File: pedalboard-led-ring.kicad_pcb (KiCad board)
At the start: 2 copper layers, 24 x 24 mm, 33 parts, among them J1 middle, J2 edge

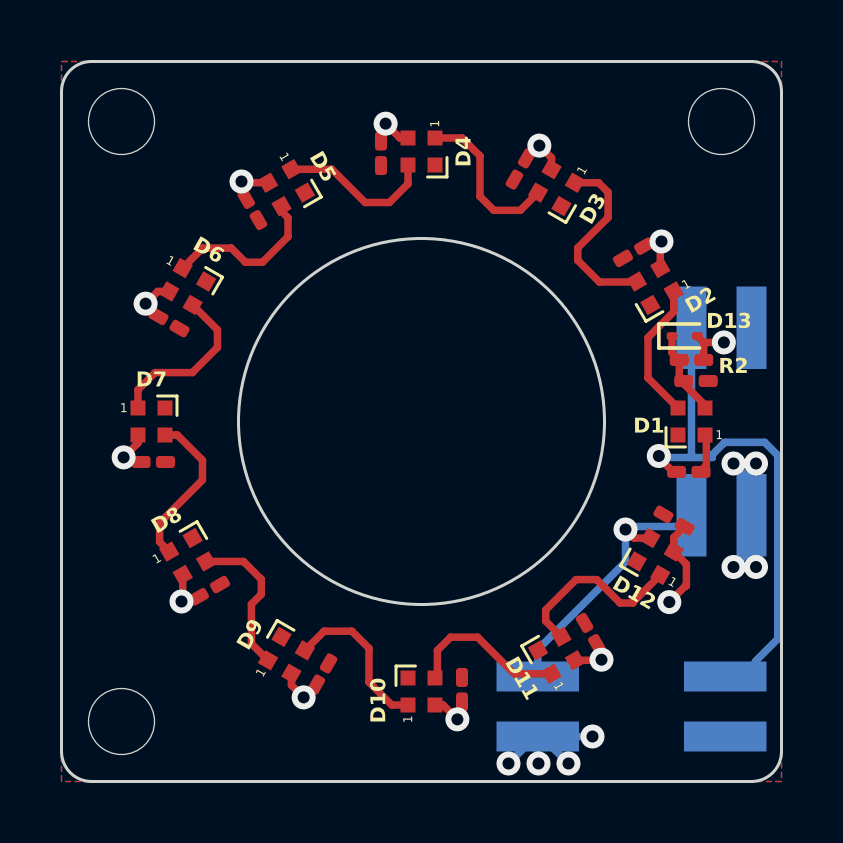
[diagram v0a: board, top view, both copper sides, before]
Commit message: Simplificaitons
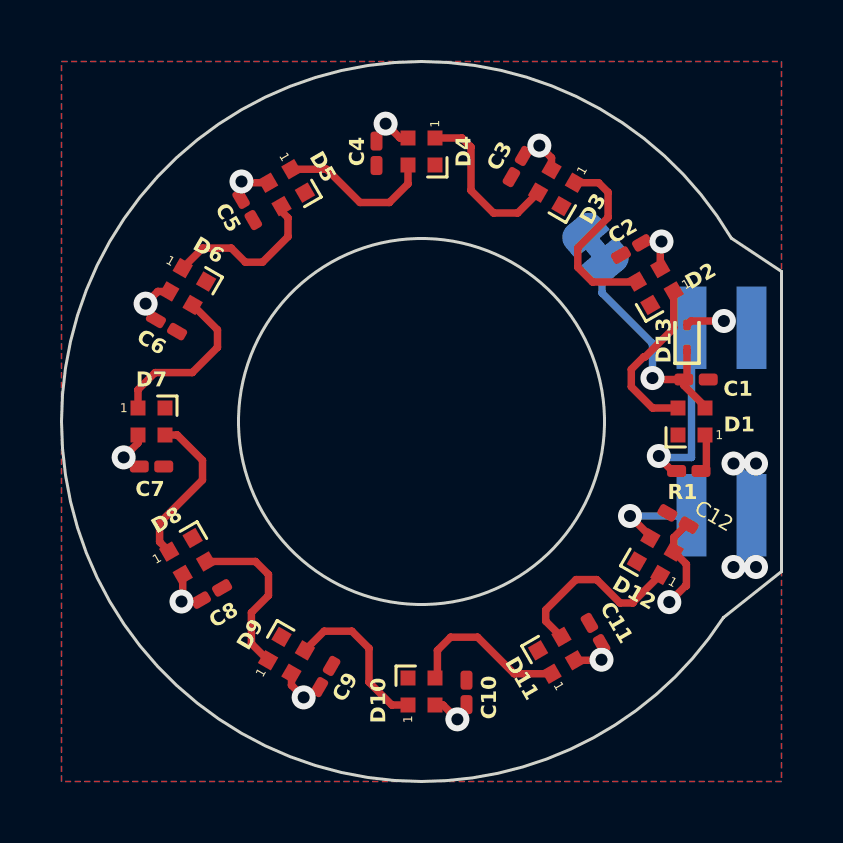
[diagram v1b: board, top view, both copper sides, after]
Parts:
- removed H1, H2, H3: MountingHole, MountingHole:MountingHole_2.2mm_M2
- removed J2: edge, Connector_PinSocket_2.00mm:PinSocket_2x02_P2.00mm_Vertical_SMD
- removed R2: 0, Resistor_SMD:R_0201_0603Metric_Pad0.64x0.40mm_HandSolder
- added JP1: SJ, Jumper:SolderJumper-2_P1.3mm_Bridged_RoundedPad1.0x1.5mm, B.Cu at (85.8, 54.2)
- moved C10 0.17 mm to (81.5, 69.0)
- moved C5 0.17 mm to (74.2, 52.9)
- moved C7 0.16 mm to (71.0, 61.5)
- moved C11 0.16 mm to (85.8, 67.1)
- moved C4 0.15 mm to (78.5, 51.1)
- moved C12 0.14 mm to (88.5, 63.2)
- moved C6 0.13 mm to (71.5, 56.8)
- moved C9 0.13 mm to (76.8, 68.5)
- moved C3 0.13 mm to (83.2, 51.5)
- moved C2 0.13 mm to (87.0, 54.2)
- moved C8 0.13 mm to (73.0, 65.8)
- moved D13 0.09 mm to (88.8, 57.2), turned to 90 degrees
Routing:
- net Net-(J1-Pin_3): track 16.6 -> 6.09 mm
- net Net-(D12-DOUT): track 8.93 -> 3.08 mm
- net GND: track 11.3 -> 5.97 mm, vias 8 -> 4
- net Net-(D1-VDD): track 2.76 -> 7.63 mm, vias 0 -> 1
- net Net-(D1-DOUT): track 4.66 -> 5.64 mm
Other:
- outline, holes or cut-outs redrawn
- board text removed: "DO"
